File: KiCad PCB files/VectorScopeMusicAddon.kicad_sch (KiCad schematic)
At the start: 13 parts, among them J1 Conn_01x09_Socket, J3 AudioJack3_SwitchTR, SW1 SW_Push_DPDT, SW2 SW_Push_DPDT, U1 OPA2192

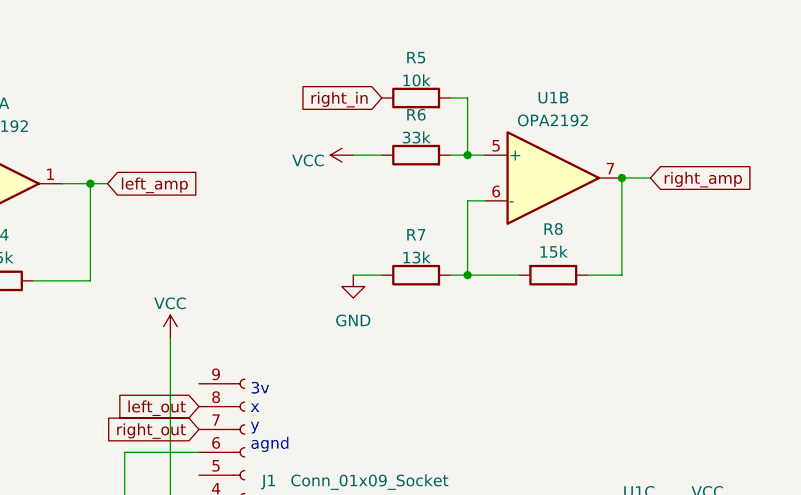
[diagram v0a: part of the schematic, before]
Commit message: inverted y-channel
changed y-channel to be inverted by differential amplifier
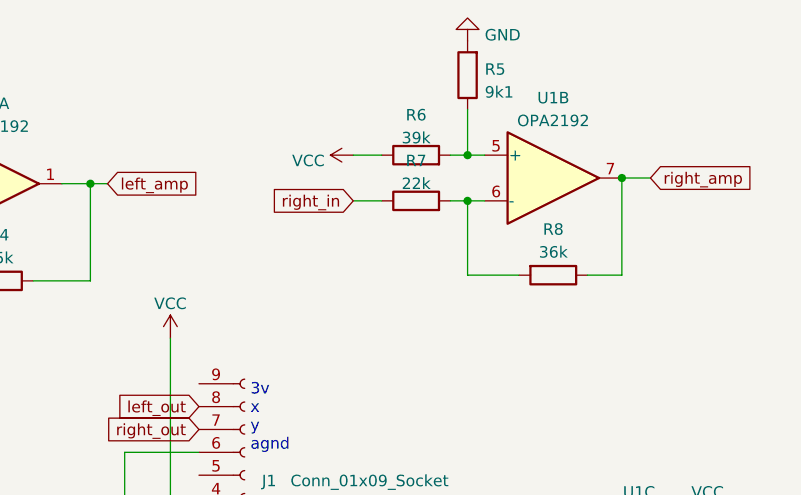
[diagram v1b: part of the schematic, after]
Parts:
- R5: value 10k -> 9k1
- R6: value 33k -> 39k
- R7: value 13k -> 22k
- R8: value 15k -> 36k
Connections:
- net GND: now also R5.2; no longer R7.1
- net right_in: now also R7.1; no longer R5.1
- net at R6.2, U1.5 (+): now also R5.1; no longer R5.2
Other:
- moved on the sheet: R5, R7
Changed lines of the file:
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@@
 (kicad_sch (version 20230121) (generator eeschema)
   (paper "A4")
+  (junction (at 156.21 37.465) (diameter 0) (color 0 0 0 0)
+  )
   (junction (at 93.98 46.355) (diameter 0) (color 0 0 0 0)
   )
-  (junction (at 156.21 45.72) (diameter 0) (color 0 0 0 0)
-  )
   (junction (at 114.3 35.56) (diameter 0) (color 0 0 0 0)
   )
@@
     (stroke (width 0) (type default))
   )
-  (wire (pts (xy 143.51 45.72) (xy 146.685 45.72))
+  (wire (pts (xy 143.51 37.465) (xy 146.685 37.465))
     (stroke (width 0) (type default))
   )
@@
     (stroke (width 0) (type default))
   )
-  (wire (pts (xy 154.305 26.035) (xy 156.21 26.035))
-    (stroke (width 0) (type default))
-  )
   (wire (pts (xy 93.98 33.02) (xy 92.075 33.02))
     (stroke (width 0) (type default))
@@
     (stroke (width 0) (type default))
   )
-  (wire (pts (xy 156.21 26.035) (xy 156.21 32.385))
-    (stroke (width 0) (type default))
-  )
   (wire (pts (xy 126.365 75.565) (xy 115.57 75.565))
     (stroke (width 0) (type default))
@@
     (stroke (width 0) (type default))
   )
+  (wire (pts (xy 156.21 27.305) (xy 156.21 32.385))
+    (stroke (width 0) (type default))
+  )
   (wire (pts (xy 169.545 45.72) (xy 173.355 45.72))
     (stroke (width 0) (type default))
@@
     (stroke (width 0) (type default))
   )
-  (wire (pts (xy 154.305 45.72) (xy 156.21 45.72))
+  (wire (pts (xy 154.305 37.465) (xy 156.21 37.465))
     (stroke (width 0) (type default))
   )
@@
     )
   )
-  (global_label "right_in" (shape input) (at 146.685 26.035 180) (fields_autoplaced)
-    (effects (font (size 1.27 1.27)) (justify right))
-    (property "Intersheetrefs" "${INTERSHEET_REFS}" (at 136.6431 26.035 0)
+  (global_label "right_in" (shape input) (at 143.51 37.465 180) (fields_autoplaced)
+    (effects (font (size 1.27 1.27)) (justify right))
+    (property "Intersheetrefs" "${INTERSHEET_REFS}" (at 133.4681 37.465 0)
       (effects (font (size 1.27 1.27)) (justify right) hide)
     )
@@
       (effects (font (size 1.27 1.27)))
     )
-    (property "Value" "15k" (at 165.735 43.18 90)
+    (property "Value" "36k" (at 165.735 43.18 90)
       (effects (font (size 1.27 1.27)))
     )
@@
     )
   )
-  (symbol (lib_id "Device:R") (at 150.495 45.72 90) (unit 1)
-    (in_bom yes) (on_board yes) (dnp no) (fields_autoplaced)
-    (property "Reference" "R7" (at 150.495 41.275 90)
-      (effects (font (size 1.27 1.27)))
-    )
-    (property "Value" "13k" (at 150.495 43.815 90)
-      (effects (font (size 1.27 1.27)))
-    )
-    (property "Footprint" "Resistor_SMD:R_0603_1608Metric_Pad0.98x0.95mm_HandSolder" (at 150.495 47.498 90)
-      (effects (font (size 1.27 1.27)) hide)
-    )
-    (property "Datasheet" "~" (at 150.495 45.72 0)
+  (symbol (lib_id "Device:R") (at 150.495 37.465 90) (unit 1)
+    (in_bom yes) (on_board yes) (dnp no) (fields_autoplaced)
+    (property "Reference" "R7" (at 150.495 33.02 90)
+      (effects (font (size 1.27 1.27)))
+    )
+    (property "Value" "22k" (at 150.495 35.56 90)
+      (effects (font (size 1.27 1.27)))
+    )
+    (property "Footprint" "Resistor_SMD:R_0603_1608Metric_Pad0.98x0.95mm_HandSolder" (at 150.495 39.243 90)
+      (effects (font (size 1.27 1.27)) hide)
+    )
+    (property "Datasheet" "~" (at 150.495 37.465 0)
       (effects (font (size 1.27 1.27)) hide)
     )
@@
       (effects (font (size 1.27 1.27)))
     )
-    (property "Value" "33k" (at 150.495 30.48 90)
+    (property "Value" "39k" (at 150.495 30.48 90)
       (effects (font (size 1.27 1.27)))
     )
@@
     )
   )
-  (symbol (lib_id "Device:R") (at 150.495 26.035 90) (unit 1)
-    (in_bom yes) (on_board yes) (dnp no) (fields_autoplaced)
-    (property "Reference" "R5" (at 150.495 21.59 90)
-      (effects (font (size 1.27 1.27)))
-    )
-    (property "Value" "10k" (at 150.495 24.13 90)
-      (effects (font (size 1.27 1.27)))
-    )
-    (property "Footprint" "Resistor_SMD:R_0603_1608Metric_Pad0.98x0.95mm_HandSolder" (at 150.495 27.813 90)
-      (effects (font (size 1.27 1.27)) hide)
-    )
-    (property "Datasheet" "~" (at 150.495 26.035 0)
+  (symbol (lib_id "Device:R") (at 156.21 23.495 180) (unit 1)
+    (in_bom yes) (on_board yes) (dnp no) (fields_autoplaced)
+    (property "Reference" "R5" (at 158.115 22.86 0)
+      (effects (font (size 1.27 1.27)) (justify right))
+    )
+    (property "Value" "9k1" (at 158.115 25.4 0)
+      (effects (font (size 1.27 1.27)) (justify right))
+    )
+    (property "Footprint" "Resistor_SMD:R_0603_1608Metric_Pad0.98x0.95mm_HandSolder" (at 157.988 23.495 90)
+      (effects (font (size 1.27 1.27)) hide)
+    )
+    (property "Datasheet" "~" (at 156.21 23.495 0)
       (effects (font (size 1.27 1.27)) hide)
     )
@@
     )
   )
-  (symbol (lib_id "power:GND") (at 143.51 45.72 0) (unit 1)
-    (in_bom yes) (on_board yes) (dnp no) (fields_autoplaced)
-    (property "Reference" "#PWR09" (at 143.51 52.07 0)
-      (effects (font (size 1.27 1.27)) hide)
-    )
-    (property "Value" "GND" (at 143.51 50.8 0)
-      (effects (font (size 1.27 1.27)))
-    )
-    (property "Footprint" "" (at 143.51 45.72 0)
-      (effects (font (size 1.27 1.27)) hide)
-    )
-    (property "Datasheet" "" (at 143.51 45.72 0)
-      (effects (font (size 1.27 1.27)) hide)
-    )
+  (symbol (lib_id "power:GND") (at 156.21 19.685 180) (unit 1)
+    (in_bom yes) (on_board yes) (dnp no) (fields_autoplaced)
+    (property "Reference" "#PWR09" (at 156.21 13.335 0)
+      (effects (font (size 1.27 1.27)) hide)
+    )
+    (property "Value" "GND" (at 158.115 19.05 0)
+      (effects (font (size 1.27 1.27)) (justify right))
+    )
+    (property "Footprint" "" (at 156.21 19.685 0)
+      (effects (font (size 1.27 1.27)) hide)
+    )
+    (property "Datasheet" "" (at 156.21 19.685 0)
+      (effects (font (size 1.27 1.27)) hide)
+    )

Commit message: Revert "inverted y-channel"
This reverts commit 5a1fcf084c13772f6a73f50f0cc3052d495043d8.
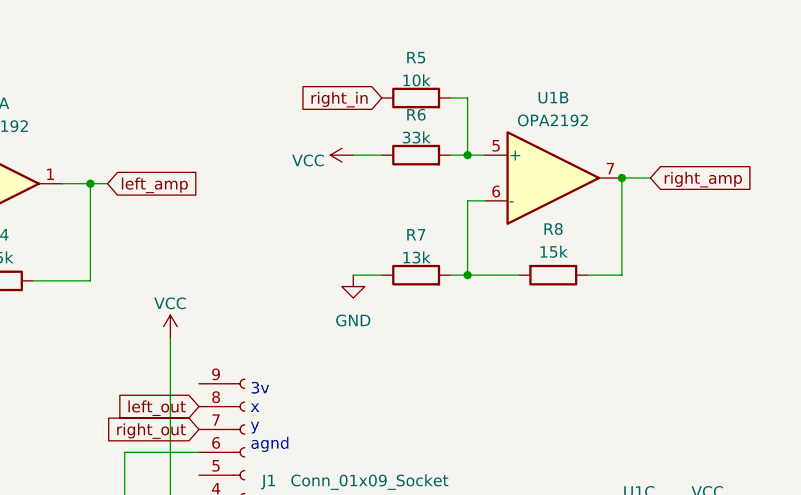
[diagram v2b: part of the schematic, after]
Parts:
- R5: value 9k1 -> 10k
- R6: value 39k -> 33k
- R7: value 22k -> 13k
- R8: value 36k -> 15k
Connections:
- net GND: now also R7.1; no longer R5.2
- net right_in: now also R5.1; no longer R7.1
- net at R6.2, U1.5 (+): now also R5.2; no longer R5.1
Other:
- moved on the sheet: R5, R7
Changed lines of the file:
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@@
 (kicad_sch (version 20230121) (generator eeschema)
   (paper "A4")
-  (junction (at 156.21 37.465) (diameter 0) (color 0 0 0 0)
-  )
   (junction (at 93.98 46.355) (diameter 0) (color 0 0 0 0)
   )
+  (junction (at 156.21 45.72) (diameter 0) (color 0 0 0 0)
+  )
   (junction (at 114.3 35.56) (diameter 0) (color 0 0 0 0)
   )
@@
     (stroke (width 0) (type default))
   )
-  (wire (pts (xy 143.51 37.465) (xy 146.685 37.465))
+  (wire (pts (xy 143.51 45.72) (xy 146.685 45.72))
     (stroke (width 0) (type default))
   )
@@
     (stroke (width 0) (type default))
   )
+  (wire (pts (xy 154.305 26.035) (xy 156.21 26.035))
+    (stroke (width 0) (type default))
+  )
   (wire (pts (xy 93.98 33.02) (xy 92.075 33.02))
     (stroke (width 0) (type default))
@@
     (stroke (width 0) (type default))
   )
+  (wire (pts (xy 156.21 26.035) (xy 156.21 32.385))
+    (stroke (width 0) (type default))
+  )
   (wire (pts (xy 126.365 75.565) (xy 115.57 75.565))
     (stroke (width 0) (type default))
@@
     (stroke (width 0) (type default))
   )
-  (wire (pts (xy 156.21 27.305) (xy 156.21 32.385))
-    (stroke (width 0) (type default))
-  )
   (wire (pts (xy 169.545 45.72) (xy 173.355 45.72))
     (stroke (width 0) (type default))
@@
     (stroke (width 0) (type default))
   )
-  (wire (pts (xy 154.305 37.465) (xy 156.21 37.465))
+  (wire (pts (xy 154.305 45.72) (xy 156.21 45.72))
     (stroke (width 0) (type default))
   )
@@
     )
   )
-  (global_label "right_in" (shape input) (at 143.51 37.465 180) (fields_autoplaced)
-    (effects (font (size 1.27 1.27)) (justify right))
-    (property "Intersheetrefs" "${INTERSHEET_REFS}" (at 133.4681 37.465 0)
+  (global_label "right_in" (shape input) (at 146.685 26.035 180) (fields_autoplaced)
+    (effects (font (size 1.27 1.27)) (justify right))
+    (property "Intersheetrefs" "${INTERSHEET_REFS}" (at 136.6431 26.035 0)
       (effects (font (size 1.27 1.27)) (justify right) hide)
     )
@@
       (effects (font (size 1.27 1.27)))
     )
-    (property "Value" "36k" (at 165.735 43.18 90)
+    (property "Value" "15k" (at 165.735 43.18 90)
       (effects (font (size 1.27 1.27)))
     )
@@
     )
   )
-  (symbol (lib_id "Device:R") (at 150.495 37.465 90) (unit 1)
-    (in_bom yes) (on_board yes) (dnp no) (fields_autoplaced)
-    (property "Reference" "R7" (at 150.495 33.02 90)
-      (effects (font (size 1.27 1.27)))
-    )
-    (property "Value" "22k" (at 150.495 35.56 90)
-      (effects (font (size 1.27 1.27)))
-    )
-    (property "Footprint" "Resistor_SMD:R_0603_1608Metric_Pad0.98x0.95mm_HandSolder" (at 150.495 39.243 90)
-      (effects (font (size 1.27 1.27)) hide)
-    )
-    (property "Datasheet" "~" (at 150.495 37.465 0)
+  (symbol (lib_id "Device:R") (at 150.495 45.72 90) (unit 1)
+    (in_bom yes) (on_board yes) (dnp no) (fields_autoplaced)
+    (property "Reference" "R7" (at 150.495 41.275 90)
+      (effects (font (size 1.27 1.27)))
+    )
+    (property "Value" "13k" (at 150.495 43.815 90)
+      (effects (font (size 1.27 1.27)))
+    )
+    (property "Footprint" "Resistor_SMD:R_0603_1608Metric_Pad0.98x0.95mm_HandSolder" (at 150.495 47.498 90)
+      (effects (font (size 1.27 1.27)) hide)
+    )
+    (property "Datasheet" "~" (at 150.495 45.72 0)
       (effects (font (size 1.27 1.27)) hide)
     )
@@
       (effects (font (size 1.27 1.27)))
     )
-    (property "Value" "39k" (at 150.495 30.48 90)
+    (property "Value" "33k" (at 150.495 30.48 90)
       (effects (font (size 1.27 1.27)))
     )
@@
     )
   )
-  (symbol (lib_id "Device:R") (at 156.21 23.495 180) (unit 1)
-    (in_bom yes) (on_board yes) (dnp no) (fields_autoplaced)
-    (property "Reference" "R5" (at 158.115 22.86 0)
-      (effects (font (size 1.27 1.27)) (justify right))
-    )
-    (property "Value" "9k1" (at 158.115 25.4 0)
-      (effects (font (size 1.27 1.27)) (justify right))
-    )
-    (property "Footprint" "Resistor_SMD:R_0603_1608Metric_Pad0.98x0.95mm_HandSolder" (at 157.988 23.495 90)
-      (effects (font (size 1.27 1.27)) hide)
-    )
-    (property "Datasheet" "~" (at 156.21 23.495 0)
+  (symbol (lib_id "Device:R") (at 150.495 26.035 90) (unit 1)
+    (in_bom yes) (on_board yes) (dnp no) (fields_autoplaced)
+    (property "Reference" "R5" (at 150.495 21.59 90)
+      (effects (font (size 1.27 1.27)))
+    )
+    (property "Value" "10k" (at 150.495 24.13 90)
+      (effects (font (size 1.27 1.27)))
+    )
+    (property "Footprint" "Resistor_SMD:R_0603_1608Metric_Pad0.98x0.95mm_HandSolder" (at 150.495 27.813 90)
+      (effects (font (size 1.27 1.27)) hide)
+    )
+    (property "Datasheet" "~" (at 150.495 26.035 0)
       (effects (font (size 1.27 1.27)) hide)
     )
@@
     )
   )
-  (symbol (lib_id "power:GND") (at 156.21 19.685 180) (unit 1)
-    (in_bom yes) (on_board yes) (dnp no) (fields_autoplaced)
-    (property "Reference" "#PWR09" (at 156.21 13.335 0)
-      (effects (font (size 1.27 1.27)) hide)
-    )
-    (property "Value" "GND" (at 158.115 19.05 0)
-      (effects (font (size 1.27 1.27)) (justify right))
-    )
-    (property "Footprint" "" (at 156.21 19.685 0)
-      (effects (font (size 1.27 1.27)) hide)
-    )
-    (property "Datasheet" "" (at 156.21 19.685 0)
-      (effects (font (size 1.27 1.27)) hide)
-    )
+  (symbol (lib_id "power:GND") (at 143.51 45.72 0) (unit 1)
+    (in_bom yes) (on_board yes) (dnp no) (fields_autoplaced)
+    (property "Reference" "#PWR09" (at 143.51 52.07 0)
+      (effects (font (size 1.27 1.27)) hide)
+    )
+    (property "Value" "GND" (at 143.51 50.8 0)
+      (effects (font (size 1.27 1.27)))
+    )
+    (property "Footprint" "" (at 143.51 45.72 0)
+      (effects (font (size 1.27 1.27)) hide)
+    )
+    (property "Datasheet" "" (at 143.51 45.72 0)
+      (effects (font (size 1.27 1.27)) hide)
+    )
